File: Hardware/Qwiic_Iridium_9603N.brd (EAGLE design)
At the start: 50.8 x 50.8 mm, 92 parts, among them J1 IRIDIUM_9603N, J10 STANDOFFS_M2X0.4_STEEL_6MM, J3 PTH, J6 ISP, J7 U.FL, J9 STANDOFFS_M2X0.4_STEEL_6MM, Q2 5.8A/30V/35mΩ, U1 ATTINY841SOIC, U2 LTC3225EDDB#TRMPBF, U3 ADM4210-1

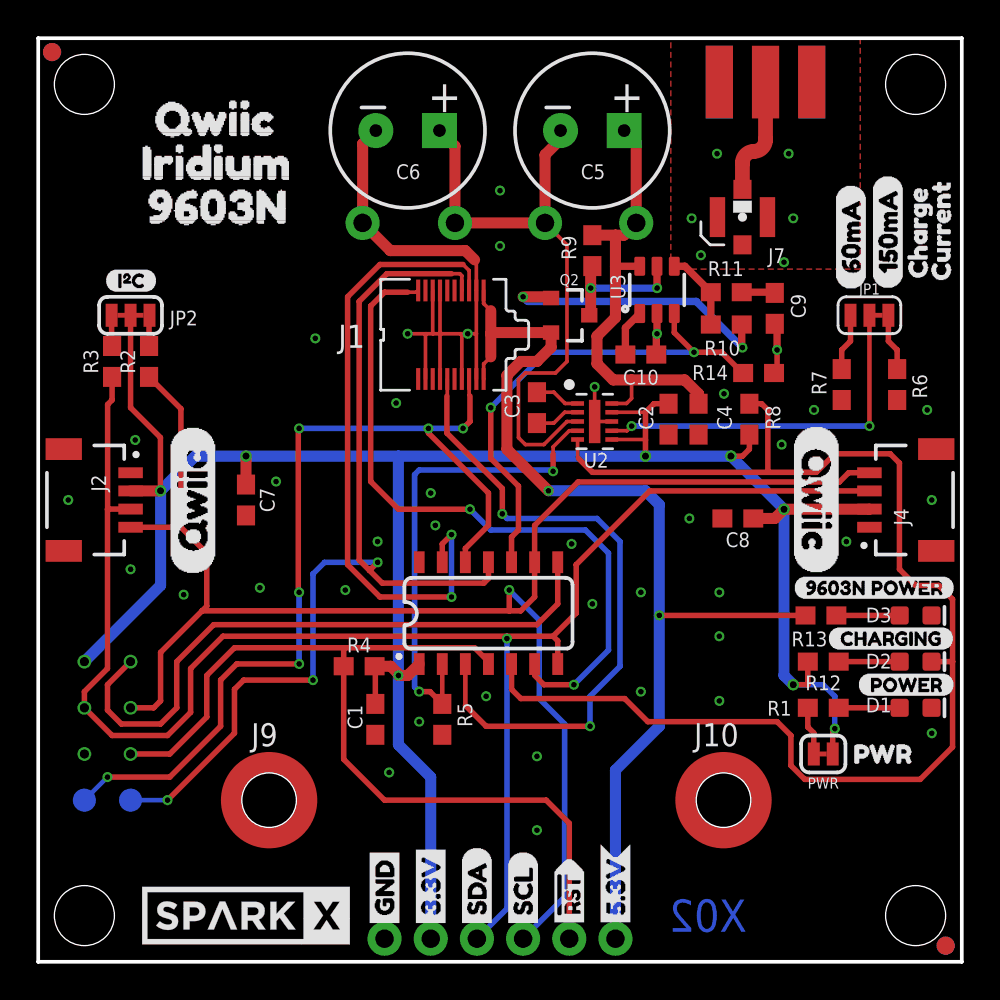
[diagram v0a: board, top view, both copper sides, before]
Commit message: Adding x02 regular and production files.
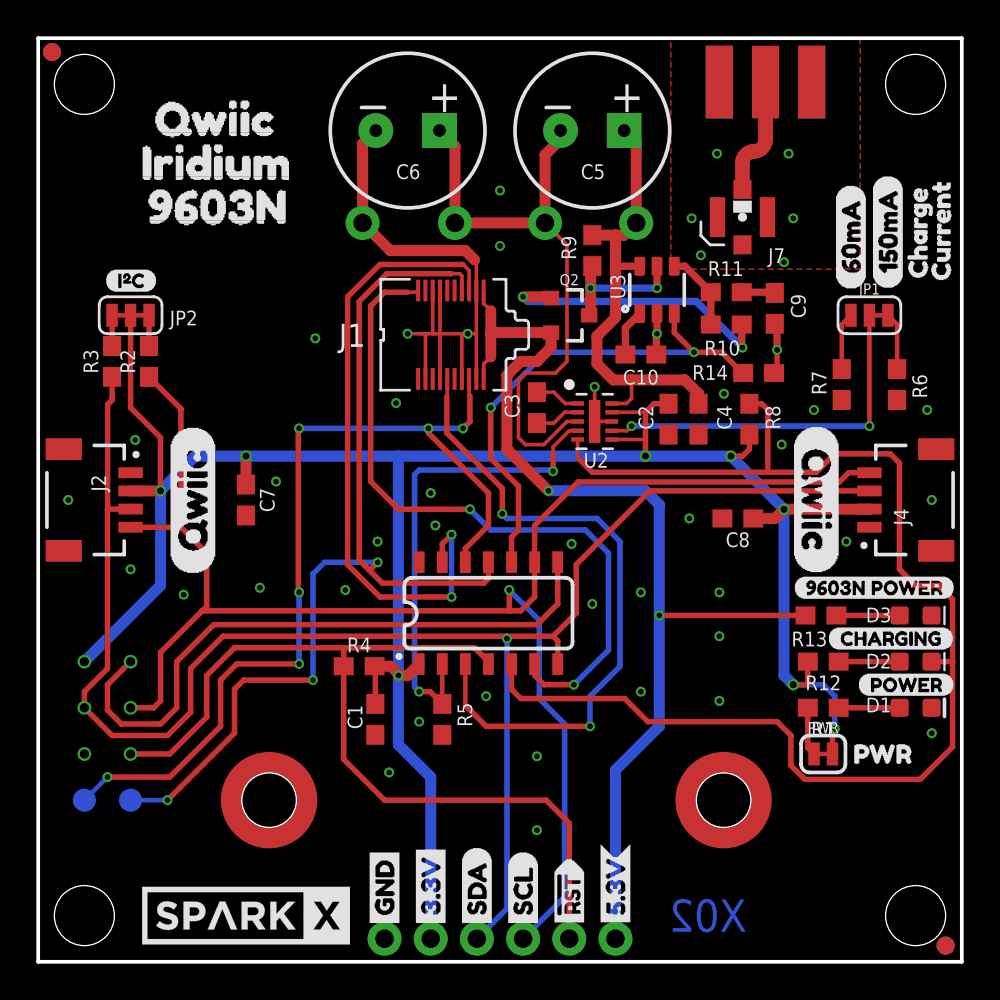
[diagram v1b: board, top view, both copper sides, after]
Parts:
- removed J10, J9: STANDOFFS_M2X0.4_STEEL_6MM, New_Parts:STANDOFF_M2X0.4
- C5, C6: device New_Parts:CPOL-RADIAL-1F-2.7V -> SparkFun-Capacitors:CPOL-RADIAL-1F-2.7V
- J1: device New_Parts:IRIDIUM_9603N -> Qwiic_Iridium_9603N:IRIDIUM_9603N
- R1, R12: device SparkFun-Resistors:0603 -> Qwiic_Iridium_9603N:0603
- R9: value 0.012R -> 0.012 Ohm; device New_Parts:0603 -> SparkFun-Resistors:0603
- U1: device New_Parts:ATTINY841 -> Qwiic_Iridium_9603N:ATTINY841
- U2: device New_Parts:DFN300X200-10L -> Qwiic_Iridium_9603N:DFN300X200-10L
- U3: device New_Parts:TSOT6 -> Qwiic_Iridium_9603N:TSOT6
- moved J1 27.5 mm to (12.7, 8.89)
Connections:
- net GND: now also J1.HOLE1, J1.HOLE2; no longer J10.1, J9.1
